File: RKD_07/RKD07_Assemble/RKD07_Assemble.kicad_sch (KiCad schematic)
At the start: 156 parts, among them J1 Conn_01x02_Socket, J10 Conn_01x04, J11 TRRS, J2 Conn_01x24, J3 Conn_01x24, J4 Conn_01x24, J5 Qwiic_RA, J6 Qwiic_RA, J7 Conn_01x06, J8 Conn_01x06, J9 Conn_01x04, SW1 SW_Push, SW10 SW_Push, SW11 SW_Push, SW12 SW_Push, SW13 SW_Push, SW14 SW_Push, SW15 SW_Push, SW16 SW_Push, SW17 SW_Push, SW18 SW_Push, SW19 SW_Push, SW2 SW_Push, SW20 SW_Push, SW21 SW_Push, SW22 SW_Push, SW23 SW_Push, SW24 SW_Push, SW25 SW_Push, SW26 SW_Push, SW27 SW_Push, SW28 SW_Push, SW29 SW_Push, SW3 SW_Push, SW30 RotaryEncoder_Switch, SW31 SW_Push, SW4 SW_Push, SW5 SW_Push, SW51 SW_Push, SW52 SW_Push, SW53 SW_Push, SW54 SW_Push, SW55 SW_Push, SW56 SW_Push, SW57 SW_Push, SW58 SW_Push, SW59 SW_Push, SW6 SW_Push, SW60 SW_Push, SW61 SW_Push, SW62 SW_Push, SW63 SW_Push, SW64 SW_Push, SW65 SW_Push, SW66 SW_Push, SW67 SW_Push, SW68 SW_Push, SW69 SW_Push, SW7 SW_Push, SW70 SW_Push, SW71 SW_Push, SW72 SW_Push, SW73 SW_Push, SW74 SW_Push, SW75 SW_Push, SW76 SW_Push, SW77 SW_Push, SW78 SW_Push, SW79 SW_Push, SW8 SW_Push, SW80 SW_Push, SW81 SW_Push, SW82 SW_Push, SW83 SW_Push, SW84 SW_Push, SW85 SW_Push, SW86 SW_Push, SW87 SW_Push, SW88 SW_Push, SW89 SW_Push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

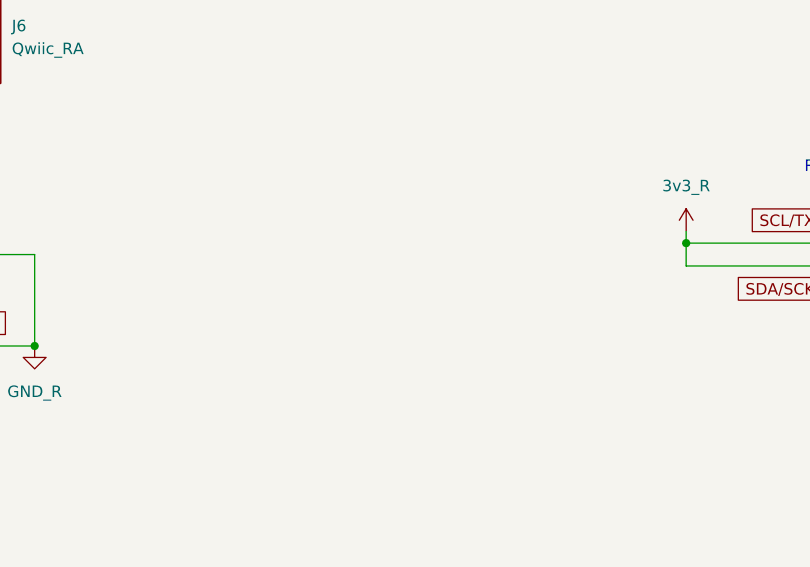
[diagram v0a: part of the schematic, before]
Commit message: 07Geek追加
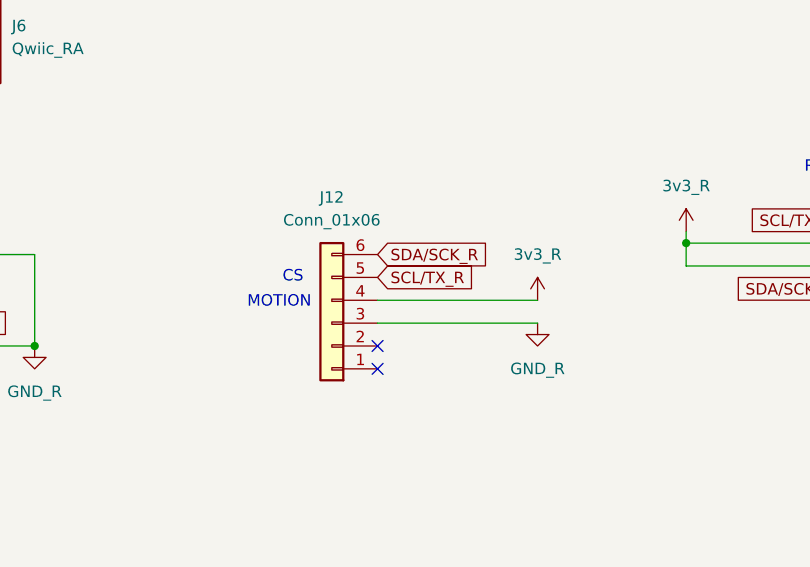
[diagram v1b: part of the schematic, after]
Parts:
- added J12: Conn_01x06, Connector_FFC-FPC:Hirose_FH12-6S-0.5SH_1x06-1MP_P0.50mm_Horizontal, symbol Connector_Generic:Conn_01x06
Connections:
- net 3v3_R: now also J12.4 (Pin_4)
- net GND_R: now also J12.3 (Pin_3)
- net SCL/TX_R: now also J12.5 (Pin_5)
- net SDA/SCK_R: now also J12.6 (Pin_6)
- no-connect marks 15 -> 17
